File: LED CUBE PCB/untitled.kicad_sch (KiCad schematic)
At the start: 29 parts, among them J1 Conn_01x04, J2 Conn_01x20, J3 Conn_01x20, SW1 RESET, Y1 8MHz, Y2 32.786KHz

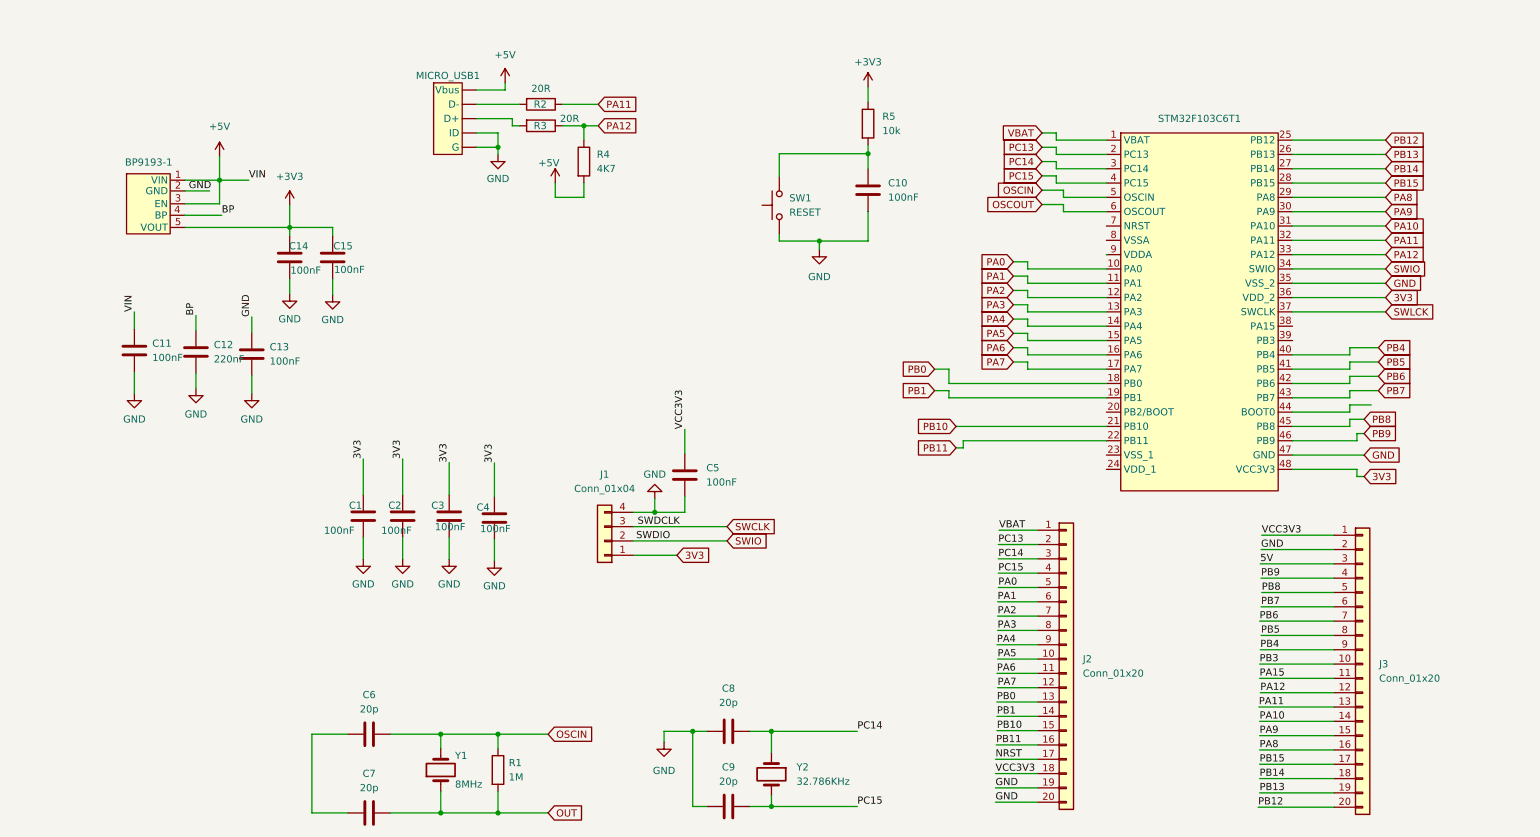
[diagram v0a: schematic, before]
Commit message: Push changes
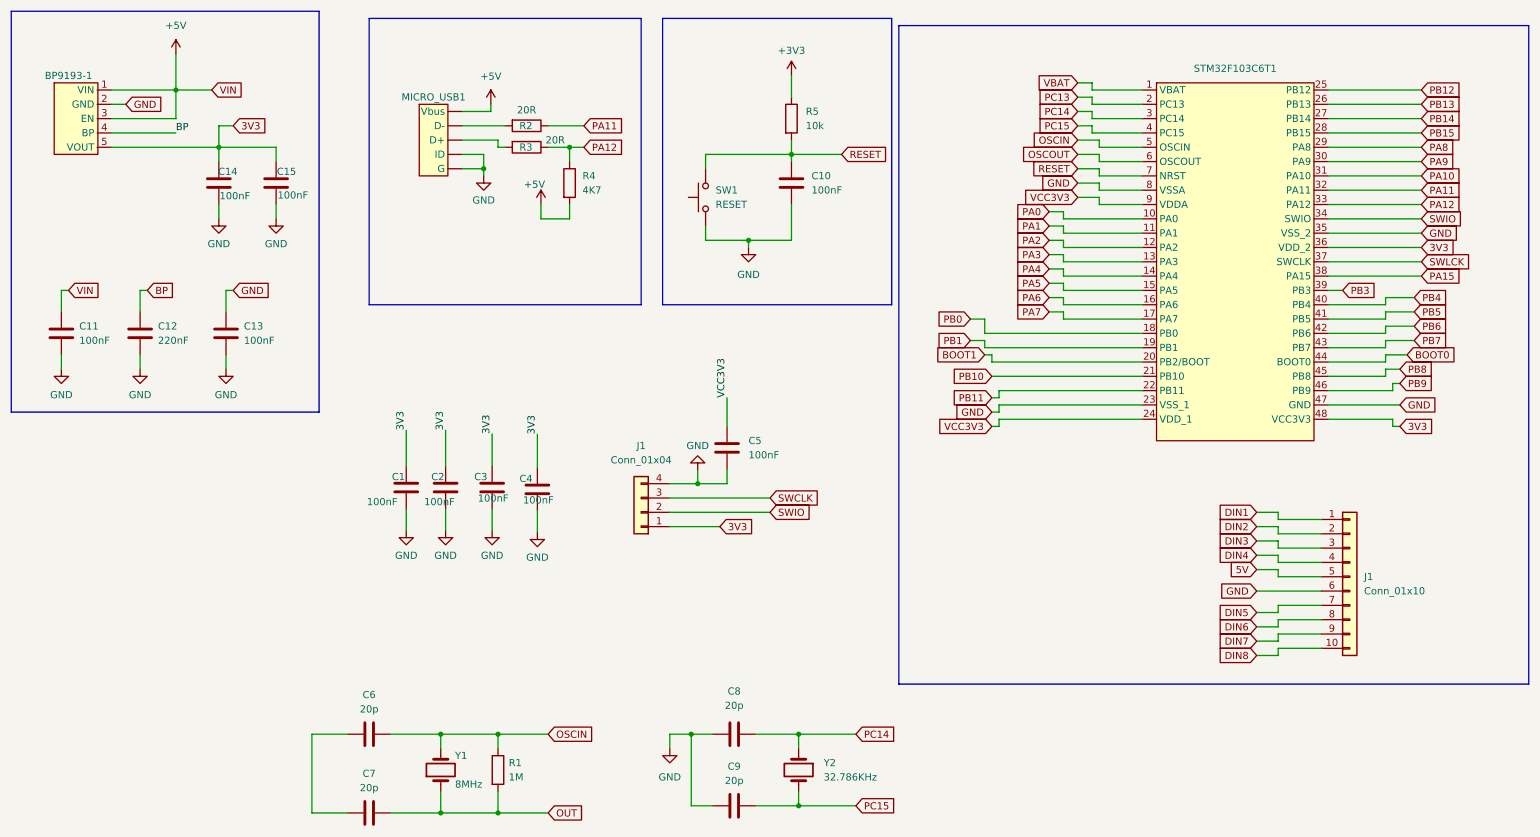
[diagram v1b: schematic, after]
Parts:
- removed J2, J3: Conn_01x20, symbol Connector_Generic:Conn_01x20
- added J1: Conn_01x10, symbol Connector_Generic:Conn_01x10
- STM32F103C6T1: footprint (none) -> STM32F103C8T6_LQFP48:STM32F103C8T6_LQFP
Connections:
- net +3V3: no longer BP9193-1.5 (VOUT), C14.1, C15.1
- net 3V3: now also BP9193-1.5 (VOUT), C14.1, C15.1, J1.1 (Pin_1)
- net 5V: now also J1.5 (Pin_5)
- net GND: now also STM32F103C6T1.23 (VSS_1), STM32F103C6T1.8 (VSSA), J1.6 (Pin_6)
- net PA15: now also STM32F103C6T1.38 (PA15)
- net PB3: now also STM32F103C6T1.39 (PB3)
- net VCC3V3: now also STM32F103C6T1.24 (VDD_1), STM32F103C6T1.9 (VDDA)
- net RESET: now reaches C10.1, R5.2, SW1.2
- net RESET: now also STM32F103C6T1.7 (NRST)
- net BOOT1: now reaches STM32F103C6T1.20 (PB2/BOOT)
- net BOOT0: now reaches STM32F103C6T1.44 (BOOT0)
- new net DIN1: J1.1 (Pin_1)
- new net DIN2: J1.2 (Pin_2)
- new net DIN3: J1.3 (Pin_3)
- new net DIN4: J1.4 (Pin_4)
- new net DIN5: J1.7 (Pin_7)
- new net DIN6: J1.8 (Pin_8)
- new net DIN7: J1.9 (Pin_9)
- new net DIN8: J1.10 (Pin_10)
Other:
- moved on the sheet: BP9193-1, C1, C10, C11, C12, C13, C14, C15, C2, C3, C4, C5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
